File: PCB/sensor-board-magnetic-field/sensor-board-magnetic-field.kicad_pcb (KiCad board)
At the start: 2 copper layers, 23.6 x 23.5 mm, 8 parts, among them U1 MAGNETIC POGO CONN., U2 MAGNETIC POGO CONN.

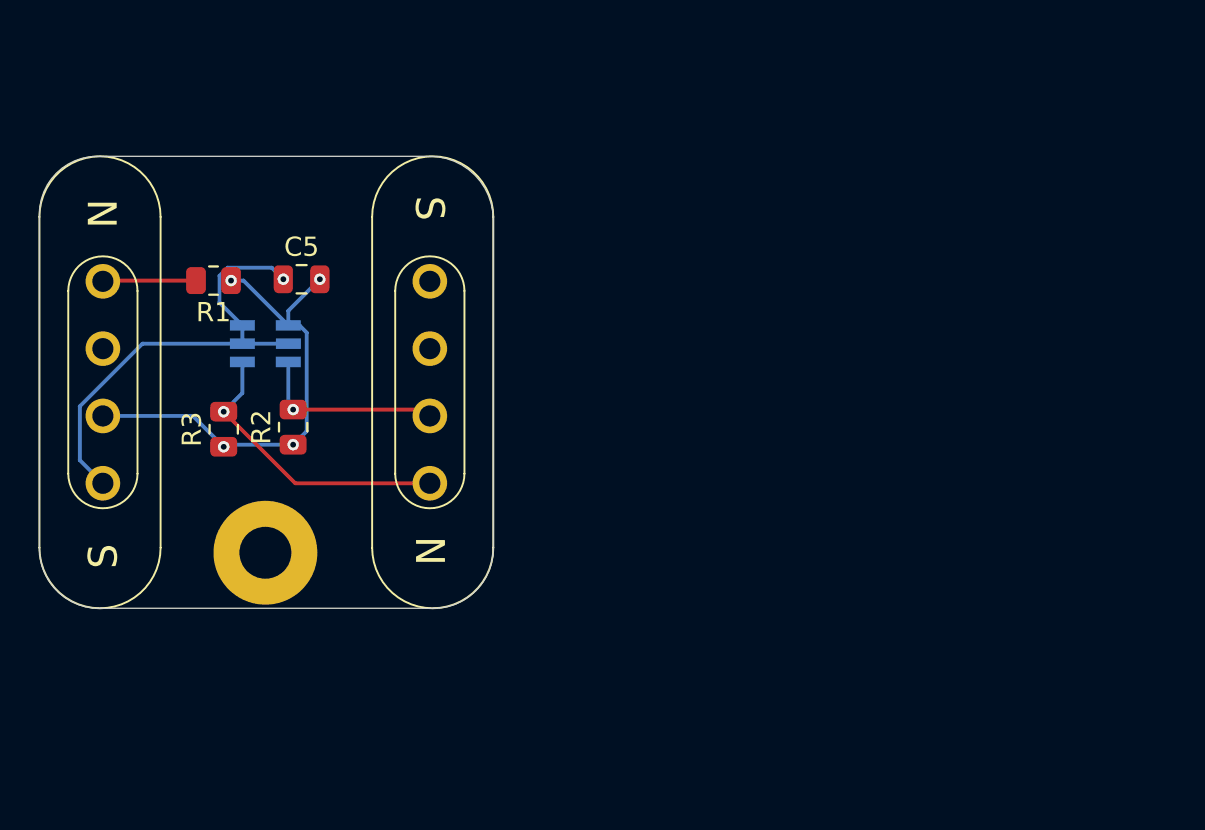
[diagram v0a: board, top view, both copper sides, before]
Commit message: made some changes
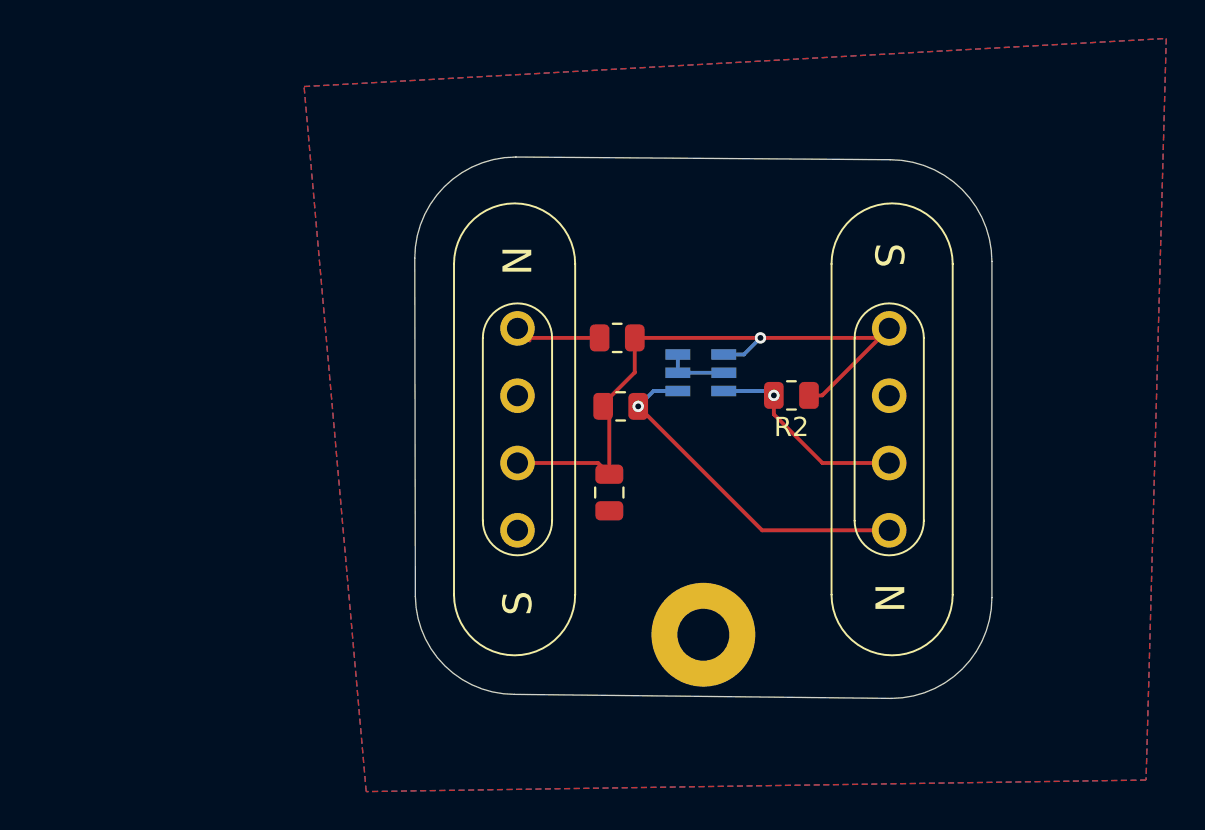
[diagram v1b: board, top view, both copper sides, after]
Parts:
- added G***: LOGO, LOGO, B.Cu at (141.7, 108.2)
- moved R2 26.0 mm to (146.2, 103.0), turned to 180 degrees
- moved U1 24.0 mm to (151.3, 104.7)
- moved H1 23.2 mm to (141.7, 115.4)
- moved TLV493D1 22.7 mm to (141.5, 101.8)
- moved U2 21.7 mm to (132.0, 104.7)
- moved R1 21.2 mm to (137.2, 100.0)
- moved R3 20.7 mm to (137.4, 103.5), turned to 0 degrees
- moved C5 19.5 mm to (136.8, 108.0), turned to 90 degrees
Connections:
- U1 pad 1: unconnected-(U1-Pad1) -> +3.3V
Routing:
- net GND: track 24.5 -> 3.34 mm, vias 1 -> 0
- net +3.3V: track 24.9 -> 34.2 mm, vias 4 -> 1
- net /SCL: track 15.2 -> 18.1 mm
- net /SDA: track 9.83 -> 10.7 mm
- net /ID: track 4.86 -> 5.37 mm
- added copper zone on B.Cu, net GND
- added copper zone on F.Cu, net GND
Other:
- board size 23.6 x 23.5 mm -> 30 x 28.1 mm
- board text added: "BOREALIS"
- board text added: "Magnetometer"
- board text removed: "Borealis Magnetometer"
